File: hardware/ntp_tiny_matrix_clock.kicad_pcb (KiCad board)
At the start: 2 copper layers, 94 x 63 mm, 96 parts, among them J1 Barrel_Jack, J10 Conn_02x04_Odd_Even, J11 Conn_02x04_Odd_Even, J12 Conn_01x04_Male, J13 Conn_01x04_Male, J2 USB_B_Micro, J3 Conn_02x04_Odd_Even, J4 Conn_02x04_Odd_Even, J5 Conn_02x04_Odd_Even, J6 Conn_02x04_Odd_Even, J7 Conn_01x06_Male, J8 Conn_02x04_Odd_Even, J9 Conn_02x04_Odd_Even, Q1 Q_NPN_BEC, Q2 AO3401, Q3 AO3401, Q4 NJL7302L-F3, Q5 Q_NPN_BEC, Q6 Q_NPN_BEC, SW1 SW_PUSH_SMALL_H, U1 PCF8563, U2 NJW4132U2-C, U3 ESP32-WROOM, U4 W256064-XALG, U5 BME280, U6 HT16D35A, U7 JW5150A, U8 HT16D35A, U9 HT16D35A

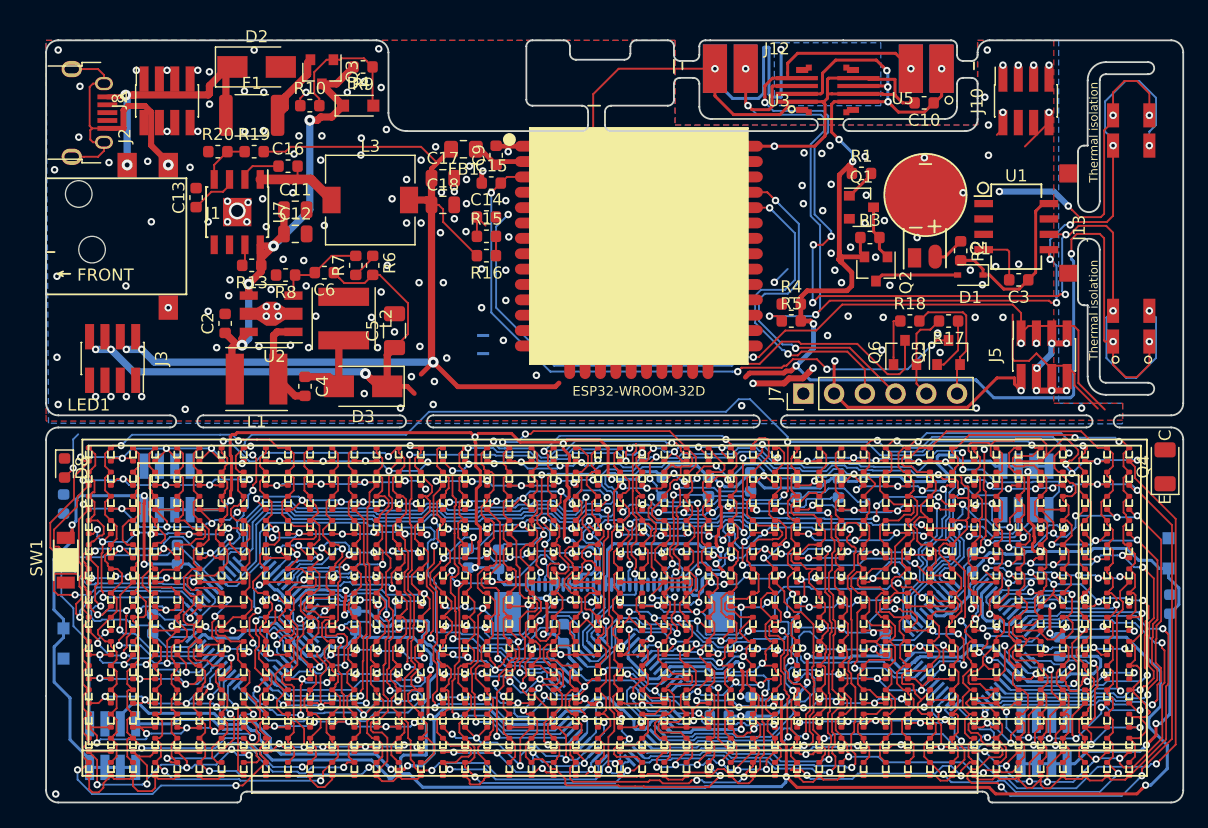
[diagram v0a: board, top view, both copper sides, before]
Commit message: Routing ongoing...
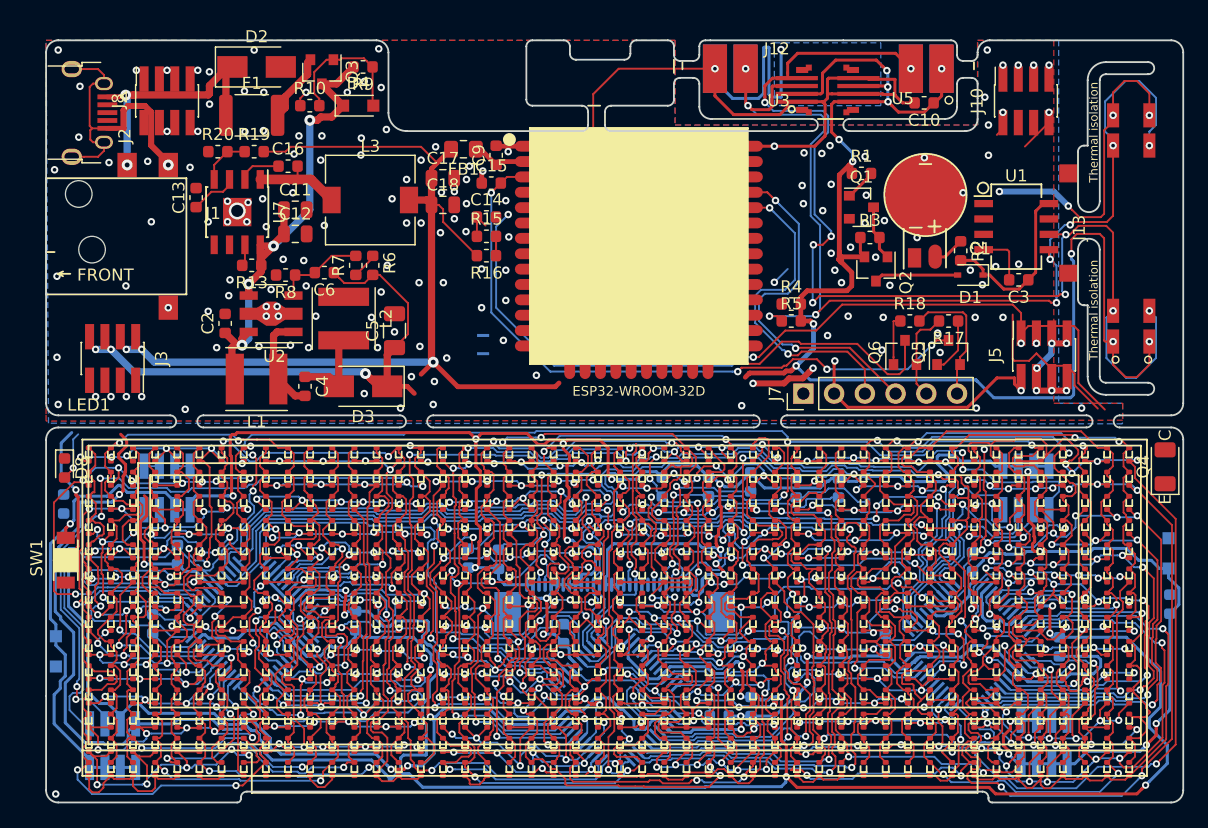
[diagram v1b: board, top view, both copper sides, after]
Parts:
- moved D6 0.91 mm to (17.8, 72.5)
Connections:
- J10 pad 1: GND -> LED_~SLAT
- J11 pad 2: GND -> LED_~SLAT
- J2 pad 2: Net-(J2-Pad2) -> (no net)
- J2 pad 3: Net-(J2-Pad3) -> (no net)
- J2 pad 4: Net-(J2-Pad4) -> (no net)
- J5 pad 1: E_AIN -> GND
- J5 pad 3: E_BUTTON -> GND
- J5 pad 5: LED_~SLAT -> GND
- J5 pad 7: STATUS -> E_AIN
- J6 pad 1: STATUS -> E_AIN
- J6 pad 3: LED_~SLAT -> GND
- J6 pad 5: E_BUTTON -> GND
- J6 pad 7: E_AIN -> GND
- J7 pad 1: Net-(J7-Pad1) -> (no net)
- J8 pad 1: /LEDVSS -> GND
- J8 pad 2: GND -> E_BUTTON
- J8 pad 3: /LEDVSS -> GND
- J8 pad 4: GND -> STATUS
- J8 pad 5: /LEDVDD -> GND
- J8 pad 7: /LEDVDD -> GND
- J9 pad 1: GND -> E_BUTTON
- J9 pad 2: /LEDVSS -> GND
- J9 pad 3: GND -> STATUS
- J9 pad 4: /LEDVSS -> GND
- J9 pad 6: /LEDVDD -> GND
- J9 pad 8: /LEDVDD -> GND
- JP1 pad 2: /LEDVDD -> (no net)
- JP2 pad 2: /LEDVSS -> (no net)
- U1 pad 1: Net-(U1-Pad1) -> (no net)
- U1 pad 2: Net-(U1-Pad2) -> (no net)
- U1 pad 3: Net-(U1-Pad3) -> (no net)
- U1 pad 7: Net-(U1-Pad7) -> (no net)
- U3 pad 10: Net-(U3-Pad10) -> (no net)
- U3 pad 11: Net-(U3-Pad11) -> (no net)
- U3 pad 12: Net-(U3-Pad12) -> (no net)
- U3 pad 13: Net-(U3-Pad13) -> (no net)
- U3 pad 14: Net-(U3-Pad14) -> (no net)
- U3 pad 16: Net-(U3-Pad16) -> (no net)
- U3 pad 17: Net-(U3-Pad17) -> (no net)
- U3 pad 18: Net-(U3-Pad18) -> (no net)
- U3 pad 19: Net-(U3-Pad19) -> (no net)
- U3 pad 20: Net-(U3-Pad20) -> (no net)
- U3 pad 21: Net-(U3-Pad21) -> (no net)
- U3 pad 22: Net-(U3-Pad22) -> (no net)
- U3 pad 23: Net-(U3-Pad23) -> (no net)
- U3 pad 24: Net-(U3-Pad24) -> (no net)
- U3 pad 28: Net-(U3-Pad28) -> (no net)
- U3 pad 32: Net-(U3-Pad32) -> (no net)
- U3 pad 33: Net-(U3-Pad33) -> (no net)
- U3 pad 36: Net-(U3-Pad36) -> (no net)
- U3 pad 37: Net-(U3-Pad37) -> (no net)
- U3 pad 4: Net-(U3-Pad4) -> (no net)
- U3 pad 6: LED_SIN -> (no net)
- U3 pad 9: Net-(U3-Pad9) -> (no net)
- U4 pad 11: Net-(U4-Pad11) -> (no net)
- U4 pad 20: Net-(U4-Pad20) -> (no net)
- U4 pad 21: Net-(U4-Pad21) -> (no net)
- U4 pad 23: Net-(U4-Pad23) -> (no net)
- U7 pad 5: Net-(U7-Pad5) -> (no net)
- U7 pad 6: Net-(U7-Pad6) -> (no net)
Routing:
- net GND: track 433.0 -> 516.9 mm, vias 207 -> 212
- net E_AIN: track 74.4 -> 2.61 mm, vias 3 -> 0
- net +12V: track 81.3 -> 143.2 mm, vias 10 -> 14
- net /LED_VDD: track 184.0 -> 220.6 mm, vias 9 -> 10
- net /LED_VSS: track 139.2 -> 166.1 mm, vias 8 -> 10
- net /k0000: track 46.1 -> 56.0 mm, vias 6 -> 9
- net /k0002: track 45.3 -> 41.1 mm, vias 6 -> 7
- net /a0001: track 90.4 -> 94.4 mm
- net /a0000: track 88.9 -> 92.2 mm
- net /a0004: track 95.6 -> 93.3 mm
- net /k0001: track 47.3 -> 45.8 mm, vias 6 -> 8
- net /a0007: track 101.8 -> 100.5 mm
- net +3V3: track 379.6 -> 380.7 mm
- net /k0215: track 73.0 -> 72.0 mm
- net /k0015: track 47.3 -> 46.4 mm
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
